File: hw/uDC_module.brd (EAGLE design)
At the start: 25 x 45 mm, 38 parts, among them J1 GROVE-4P-2.0-3470130P1, J2 GROVE-4P-2.0-3470130P1, U5 LD3985XX, X1 22-23-2021, X2 22-23-2021, X3 53047-06, X4 53047-06

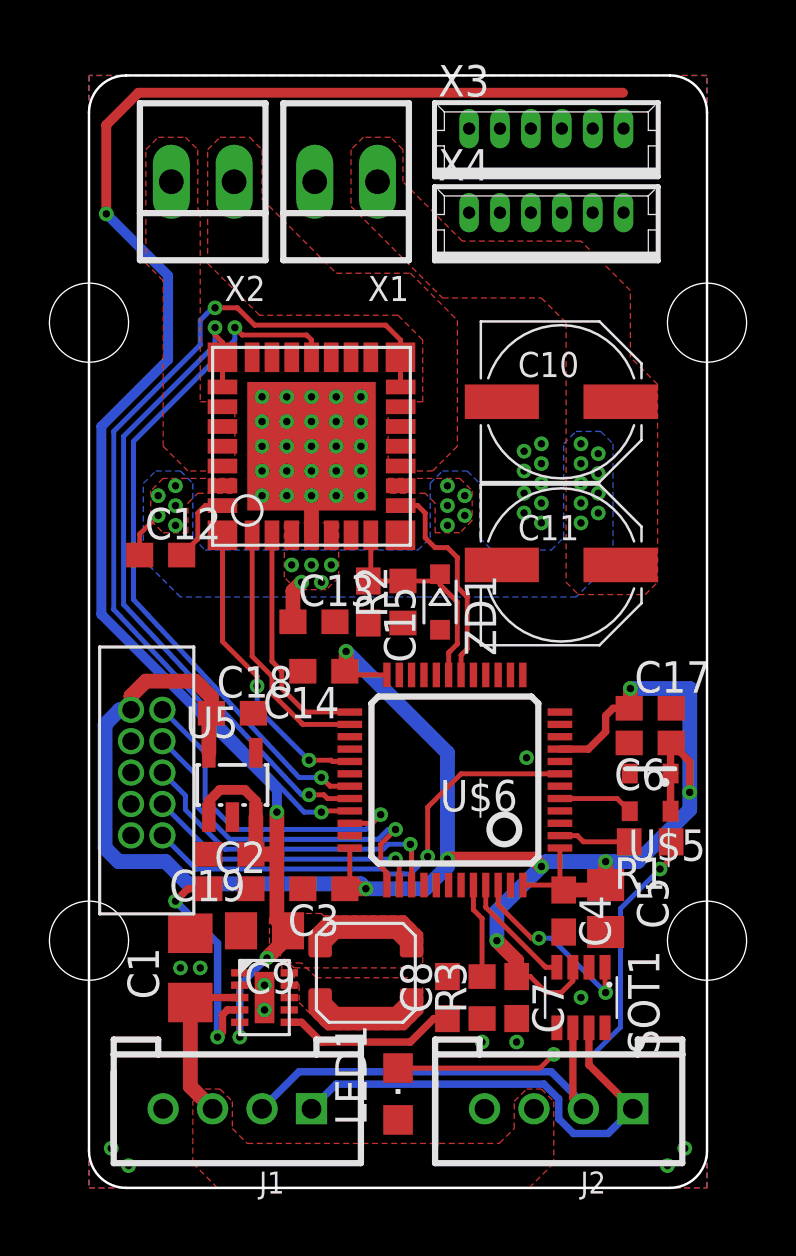
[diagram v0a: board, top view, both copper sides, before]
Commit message: layout completed
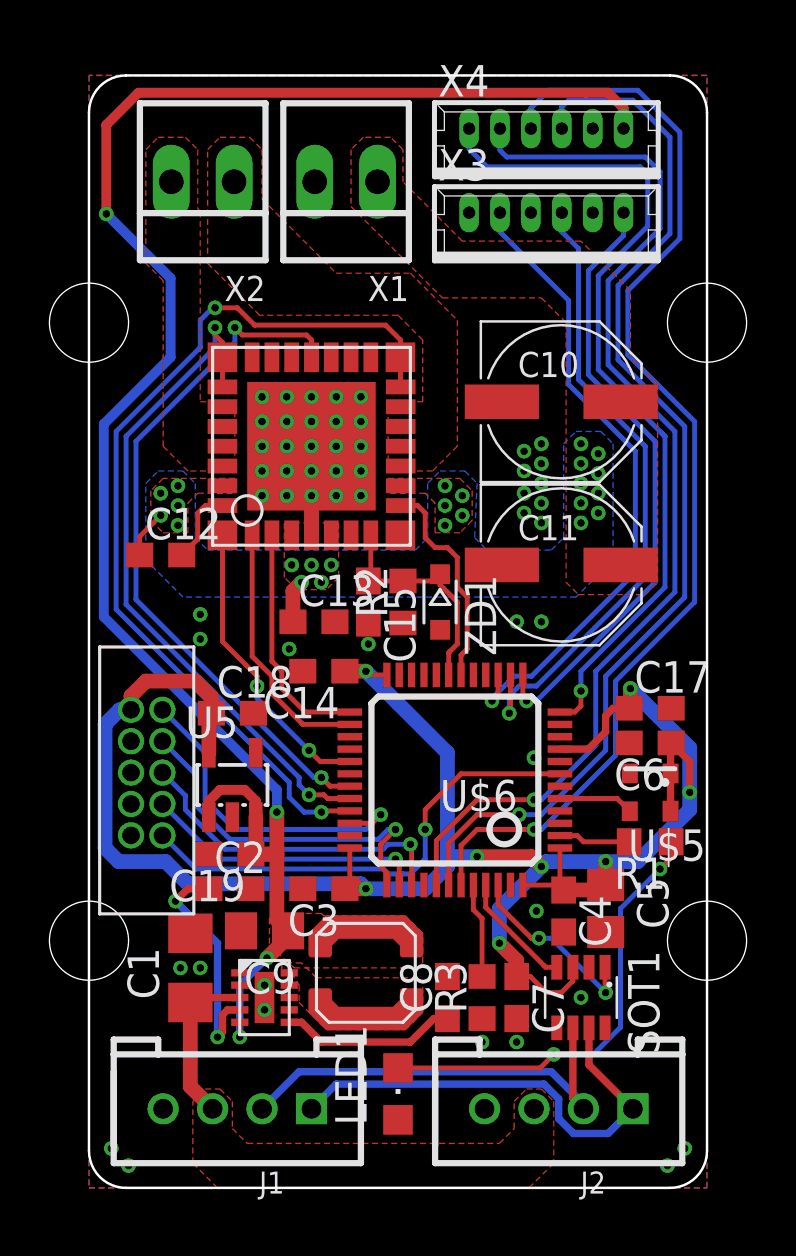
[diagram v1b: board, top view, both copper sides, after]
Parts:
- moved X3 3.40 mm to (18.5, 39.0)
- moved X4 3.40 mm to (18.5, 42.4)
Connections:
- new net ANALOG: U$6.12, X4.6
- new net ENC_A: U$6.42, X4.3
- new net ENC_B: U$6.43, X4.4
- new net ENC_I: U$6.41, X4.5
- new net LIMIT_A: U$6.13, X3.1
- new net LIMIT_B: U$6.14, X3.3
- new net STOP: U$6.15, X3.5
- net +5V: now also X4.1
- net GND: now also X3.2, X3.4, X3.6, X4.2
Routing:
- net ENC_B: track 0.00 -> 45.7 mm, vias 0 -> 1
- net ENC_I: track 0.00 -> 44.1 mm, vias 0 -> 1
- net ENC_A: track 0.00 -> 43.7 mm, vias 0 -> 1
- net ANALOG: track 0.00 -> 34.6 mm, vias 0 -> 1
- net STOP: track 0.00 -> 26.0 mm, vias 0 -> 1
- net LIMIT_B: track 0.00 -> 25.9 mm, vias 0 -> 1
- net LIMIT_A: track 0.00 -> 25.0 mm, vias 0 -> 1
- net +3V3: track 86.7 -> 83.3 mm
- net +5V: track 71.2 -> 72.3 mm
- net GND: vias 46 -> 53
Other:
- board text added: "ENC"
- board text added: "MOTOR"
- board text added: "STOP"
- board text added: "SUPPLY"
